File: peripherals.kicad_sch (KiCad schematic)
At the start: 17 parts, among them J1 1-776267-1, Q4 2N7002KT1G, Q5 2N7002KT1G, U7 LTV-827S

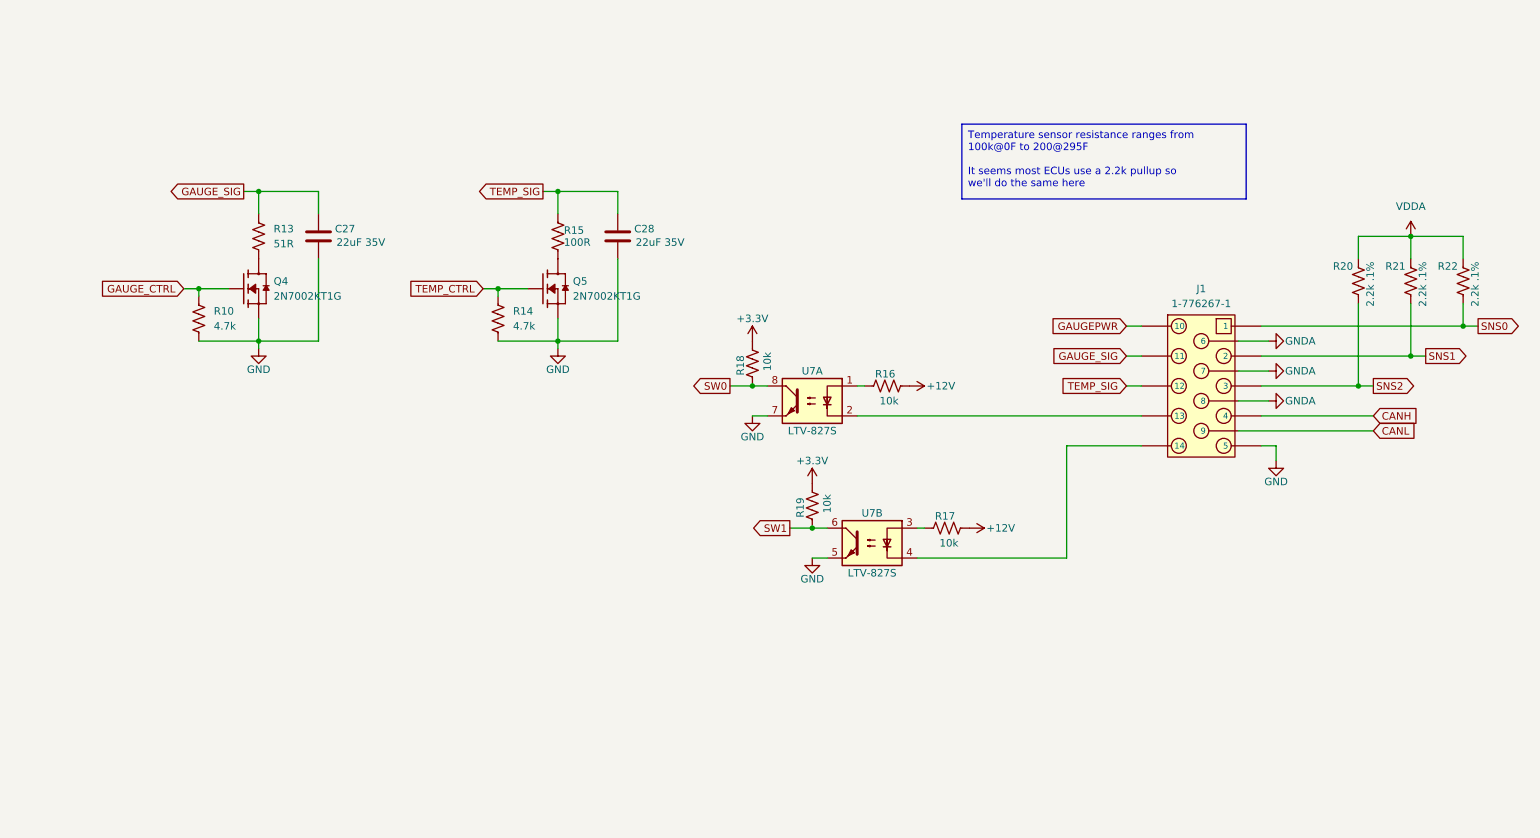
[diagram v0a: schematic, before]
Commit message: Some perpipheral changes?
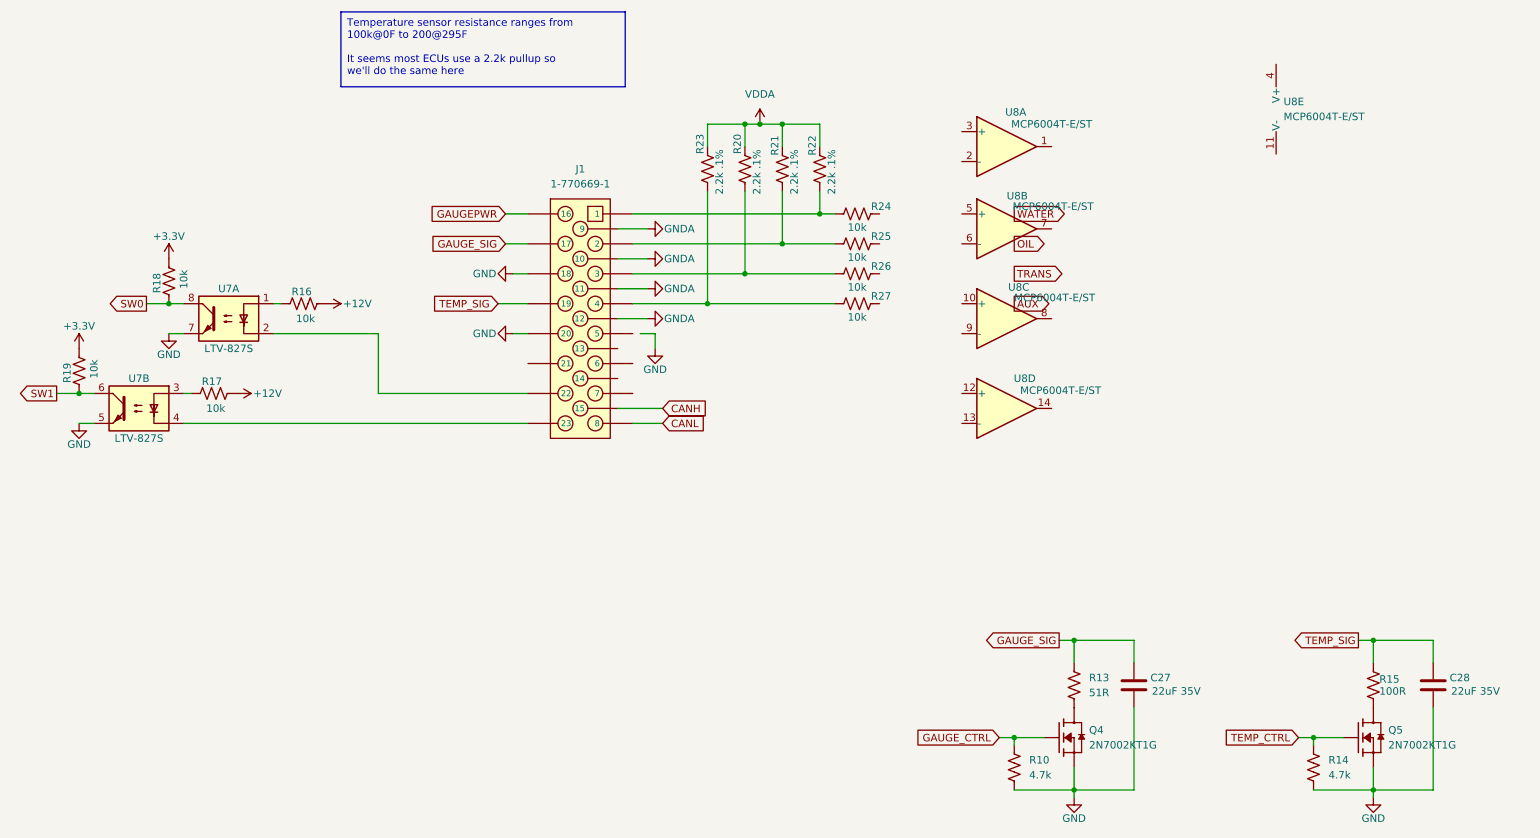
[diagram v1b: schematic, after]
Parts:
- removed J1: 1-776267-1, Sullivan-Labs:TE_1-776267-1, symbol Sullivan-Labs:CONN 14-Pin AMPSEAL RA
- added J1: 1-770669-1, Sullivan-Labs:17706691, symbol Sullivan-Labs:CONN 23-Pin AMPSEAL RA
- added R23: 2.2k .1%, Sullivan-Labs:R_0402_1005Metric, symbol Sullivan-Labs:RES_2.2k_.1%_0402
- added R24, R25, R26, R27: 10k, Sullivan-Labs:R_0402_1005Metric, symbol Sullivan-Labs:RES_10k_0402
- added U8: MCP6004T-E/ST, Sullivan-Labs:SOP65P640X120-14N, symbol Sullivan-Labs:IC 4-CH Op Amp MCP6004
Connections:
- net CANH: now also J1.15
- net CANL: now also J1.8
- net GAUGEPWR: now also J1.16
- net GAUGE_SIG: now also J1.17
- net GND: now also J1.18, J1.20
- net GNDA: now also J1.10, J1.11, J1.12, J1.9
- net TEMP_SIG: now also J1.19
- net VDDA: now also R23.1
- net at U7.2: now also J1.22
- net at U7.4: now also J1.23
- net SNS0: no longer names the net of R22.2
- net SNS0: now also J1.1, R24.1
- net SNS1: no longer names the net of R21.2
- net SNS1: now also J1.2, R25.1
- net SNS2: no longer names the net of R20.2
- net SNS2: now also J1.3, R26.1
- new net: J1.4, R23.2, R27.1
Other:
- moved on the sheet: C27, C28, Q4, Q5, R10, R13, R14, R15, R16, R17, R18, R19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
